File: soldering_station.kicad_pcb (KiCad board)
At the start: 2 copper layers, 100 x 36 mm, 110 parts, among them J1 Barrel_Jack_Switch, J2 IRON, J3 USB, J32 PROG, J5 EXT, J6 USB, Q1 BC847, Q2 Q_PMOS_GDS, Q3 MMBT2222A, Q4 BC847, SW1 Rotary_Encoder_Switch_with_Mo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, SW2 SW_SPST, SW4 RESET, U10 DS18B20, U11 ESP32-S3-WROOM-1, U2 TPS54202DDC, U3 74AHCT1G125, U4 AMS1117-3.3, U5 OPA336Nx, X1 Display_P169H002-CTP

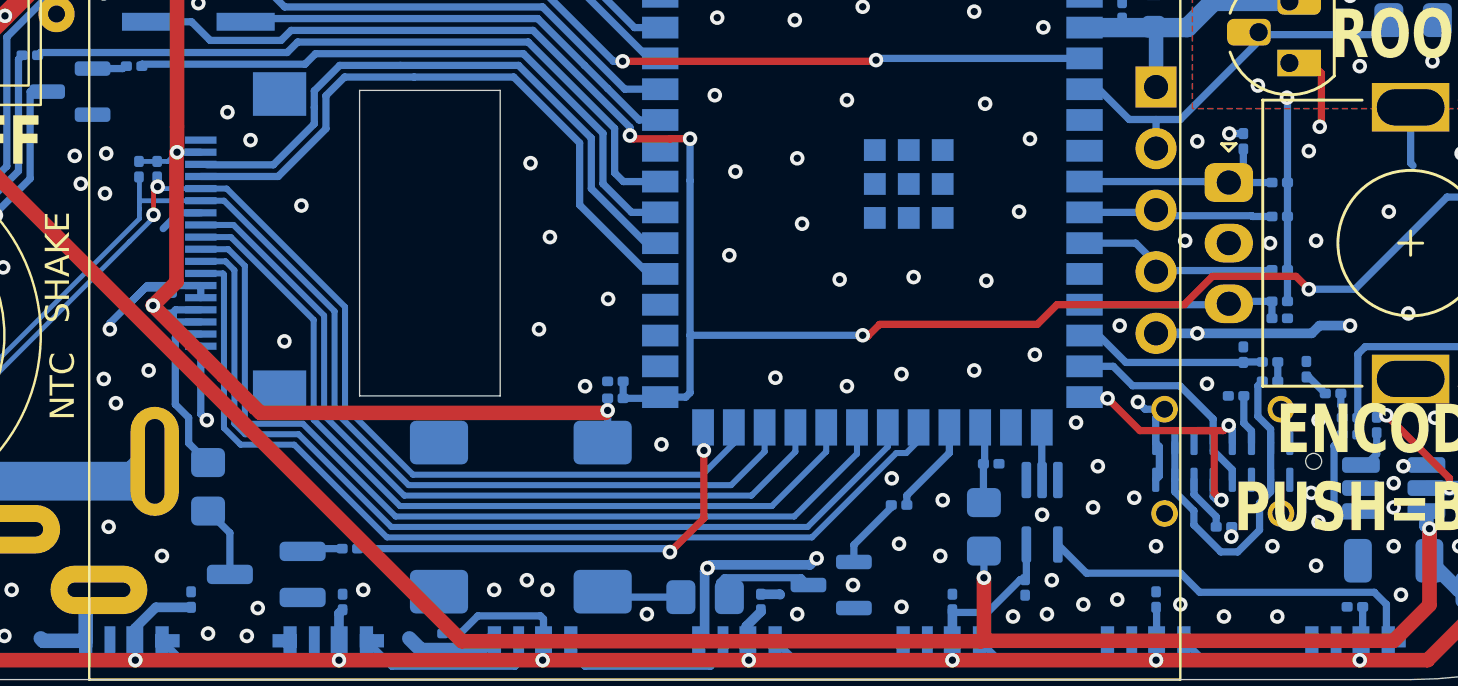
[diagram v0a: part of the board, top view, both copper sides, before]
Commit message: Layout improvements
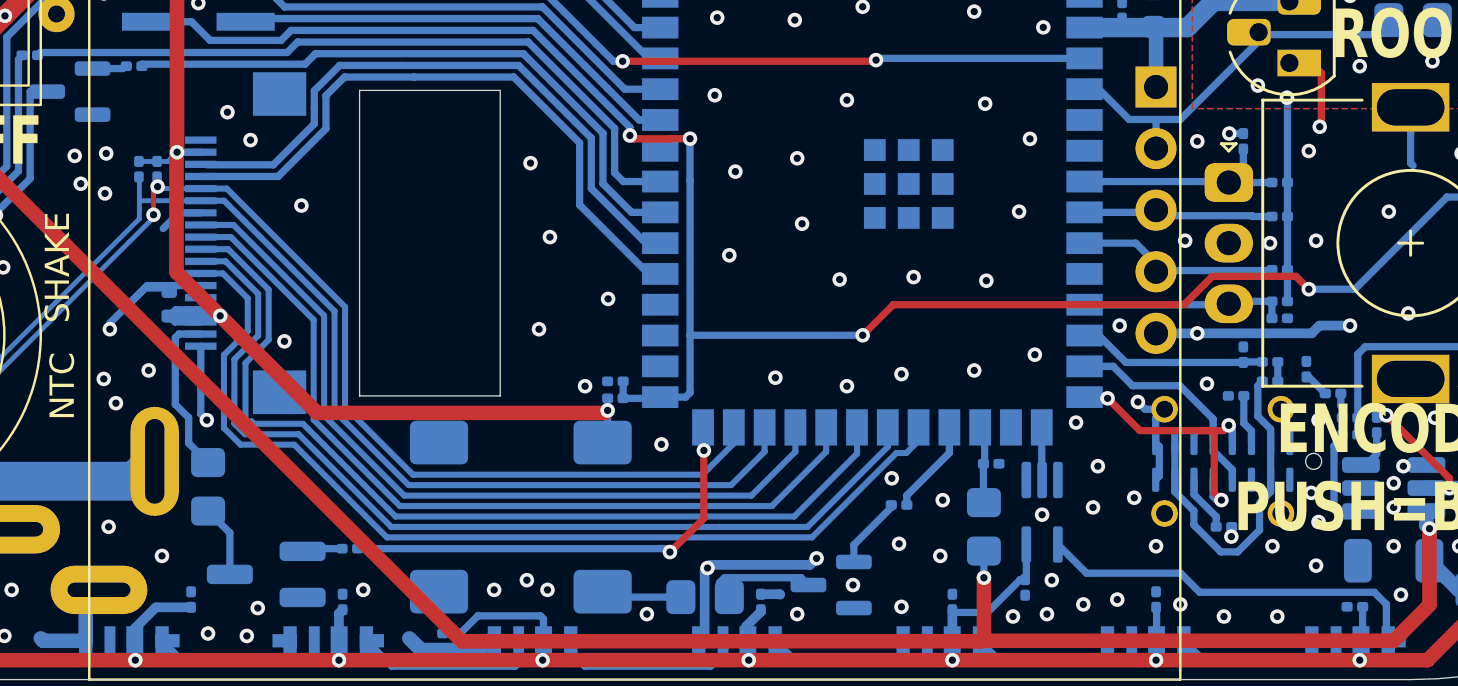
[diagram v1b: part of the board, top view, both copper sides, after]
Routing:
- net +3V3: track 172.1 -> 150.7 mm
- net LCD_SCK: track 37.5 -> 38.5 mm
- net LCD_RS: track 40.0 -> 40.8 mm
- net LCD_CS: track 38.7 -> 39.6 mm
